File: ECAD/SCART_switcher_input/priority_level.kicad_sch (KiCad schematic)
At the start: 4 parts, among them U4 74LVC1G04, U5 74LVC1G08, U6 74LVC1G08

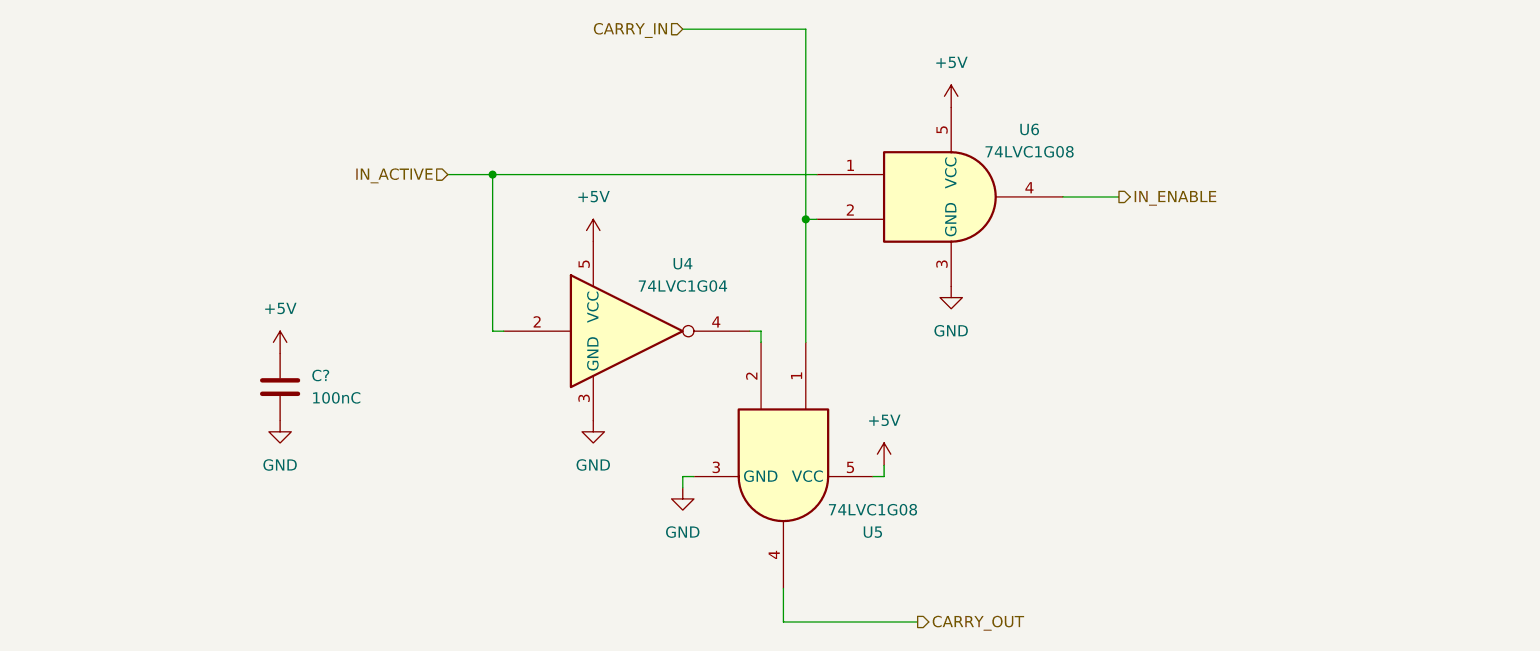
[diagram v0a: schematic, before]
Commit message: Progressed ECAD.
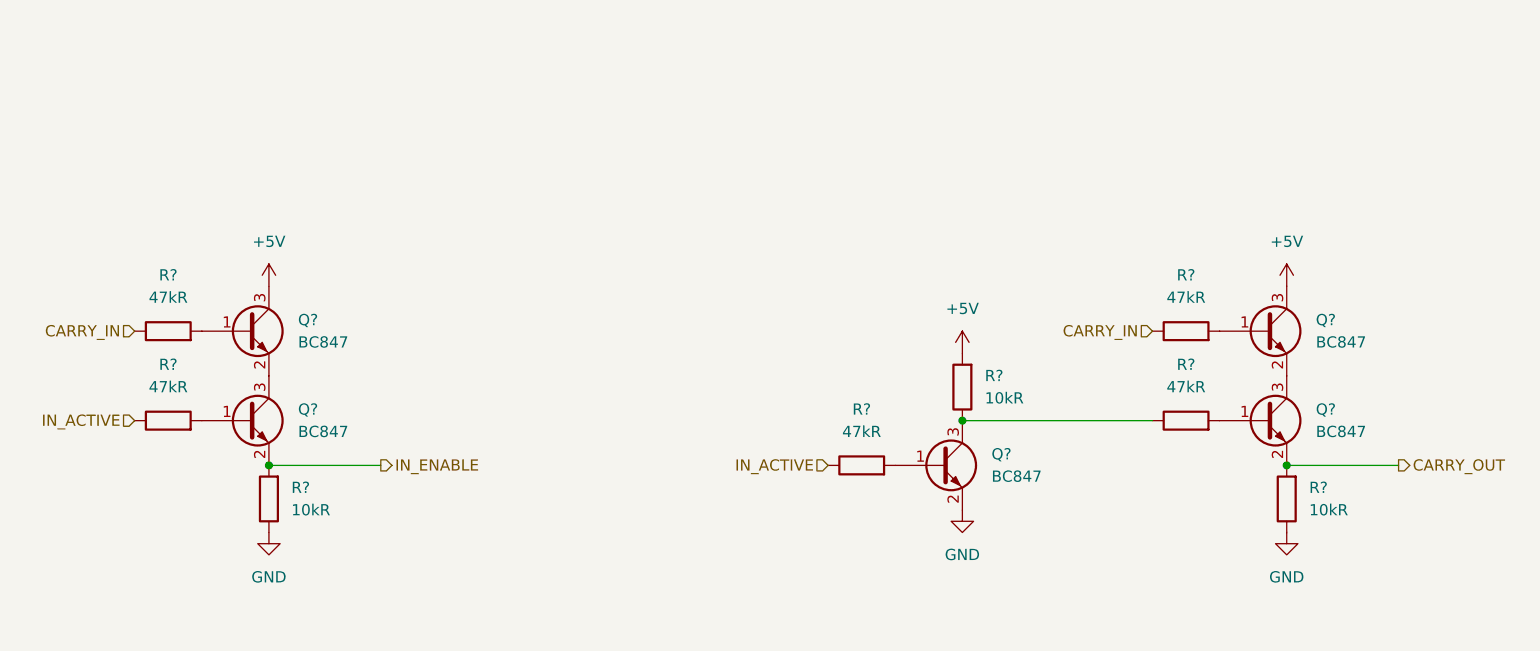
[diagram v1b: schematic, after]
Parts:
- removed C?: 100nC, Capacitor_SMD:C_0805_2012Metric, symbol Device:C
- removed U4: 74LVC1G04, Package_TO_SOT_SMD:SOT-353_SC-70-5, symbol 74xGxx:74AHC1G04
- removed U5, U6: 74LVC1G08, Package_TO_SOT_SMD:SOT-353_SC-70-5, symbol 74xGxx:74AHC1G08
- added Q? (x5): BC847, Package_TO_SOT_SMD:SOT-23, symbol Transistor_BJT:BC847
- added R? (x5): 47kR, Resistor_SMD:R_0805_2012Metric, symbol Device:R
- added R? (x3): 10kR, Resistor_SMD:R_0805_2012Metric, symbol Device:R
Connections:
- net +5V: now also Q?.3 (C), Q?.3 (C), R?.2
- net CARRY_IN: now also R?.1, R?.1
- net CARRY_OUT: now also Q?.2 (E), R?.2
- net GND: now also Q?.2 (E), R?.1, R?.1
- net IN_ACTIVE: now also R?.1, R?.1
- net IN_ENABLE: now also Q?.2 (E), R?.2
- new net: Q?.1 (B), R?.2 (x5)
- new net: Q?.2 (E), Q?.3 (C) (x2)
- new net: Q?.3 (C), R?.1, R?.1

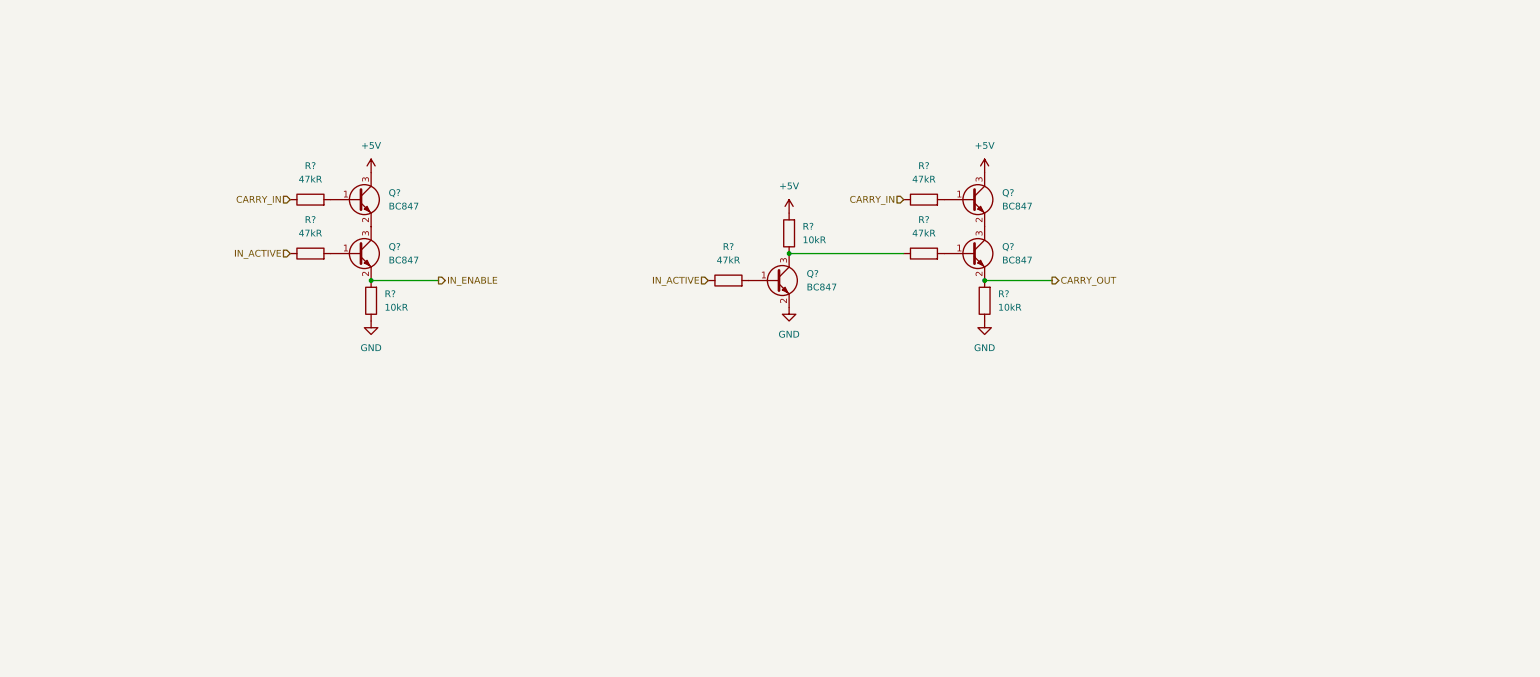
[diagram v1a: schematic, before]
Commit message: Progressed ECAD.
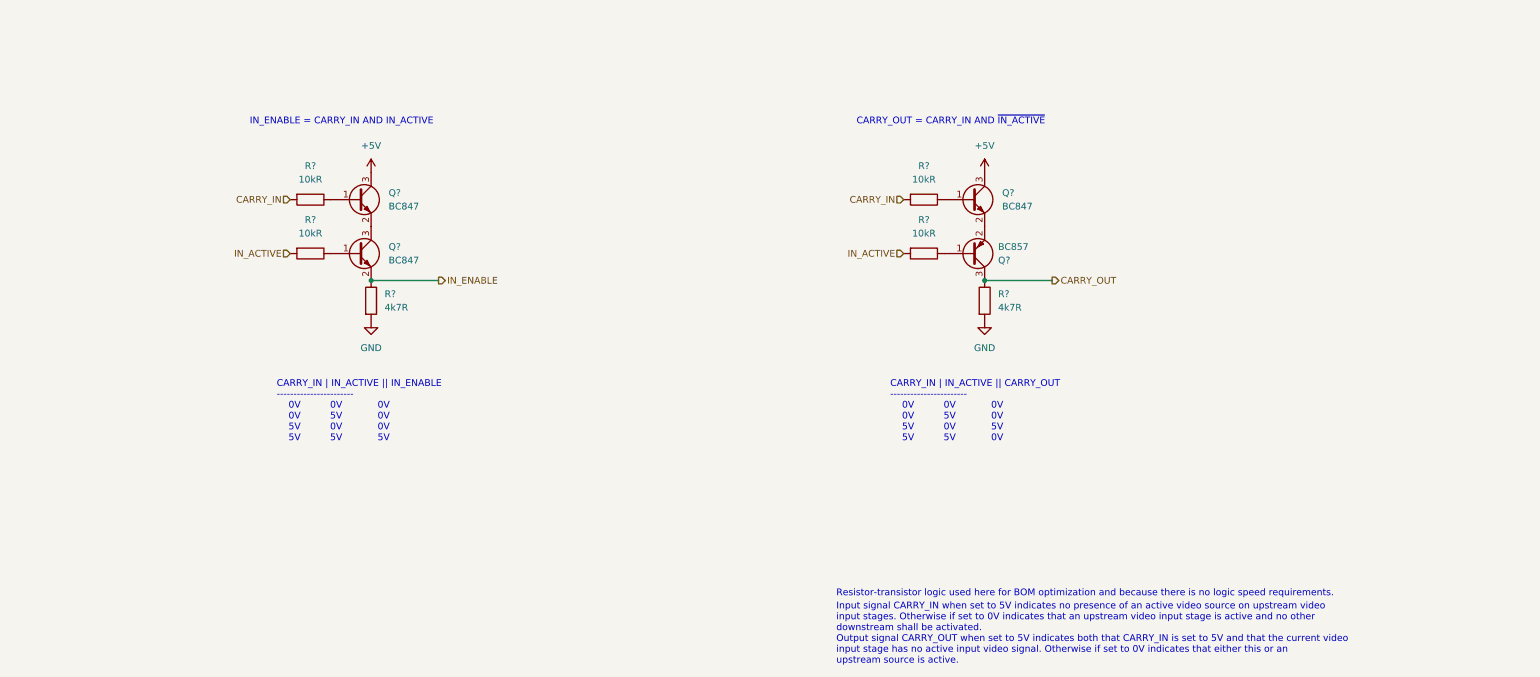
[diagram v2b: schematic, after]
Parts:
- removed Q? (x2): BC847, Package_TO_SOT_SMD:SOT-23, symbol Transistor_BJT:BC847
- removed R? (x5): 47kR, Resistor_SMD:R_0805_2012Metric, symbol Device:R
- removed R? (x3): 10kR, Resistor_SMD:R_0805_2012Metric, symbol Device:R
- added Q?: BC857, Package_TO_SOT_SMD:SOT-23, symbol Transistor_BJT:BC857
- added R? (x2): 4k7R, Resistor_SMD:R_0805_2012Metric, symbol Device:R
- added R? (x4): 10kR, Resistor_SMD:R_0805_2012Metric, symbol Device:R
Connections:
- net CARRY_IN: now also R?.2, R?.2
- net CARRY_OUT: now also Q?.3 (C), R?.1
- net GND: now also R?.2, R?.2
- net IN_ACTIVE: now also R?.2, R?.2
- net IN_ENABLE: now also R?.1
- net at Q?.1 (B): now also R?.1 (x3)
- net at Q?.2 (E): now also Q?.2 (E)
- new net: Q?.1 (B), R?.1
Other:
- note added: "CARRY_IN | IN_ACTIVE || CARRY_OUT ----------------------- 0V 0V 0V 0V 5V 0V 5V 0V 5V 5V 5V 0V"
- note added: "CARRY_IN | IN_ACTIVE || IN_ENABLE ----------------------- 0V 0V 0V 0V 5V 0V 5V 0V 0V 5V 5V 5V"
- note added: "CARRY_OUT = CARRY_IN AND ~{IN_ACTIVE}"
- note added: "IN_ENABLE = CARRY_IN AND IN_ACTIVE"
- note added: "Input signal CARRY_IN when set to 5V indicates no presence of an active video source on upstream video input stages. Otherwise if set to 0V indicates that an upstream video input stage is active and no other downstream shall be activated. Output signal CARRY_OUT when set to 5V indicates both that CARRY_IN is set to 5V and that the current video input stage has no active input video signal. Otherw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"
- note added: "Resistor-transistor logic used here for BOM optimization and because there is no logic speed requirements."

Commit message: progressed ecad.
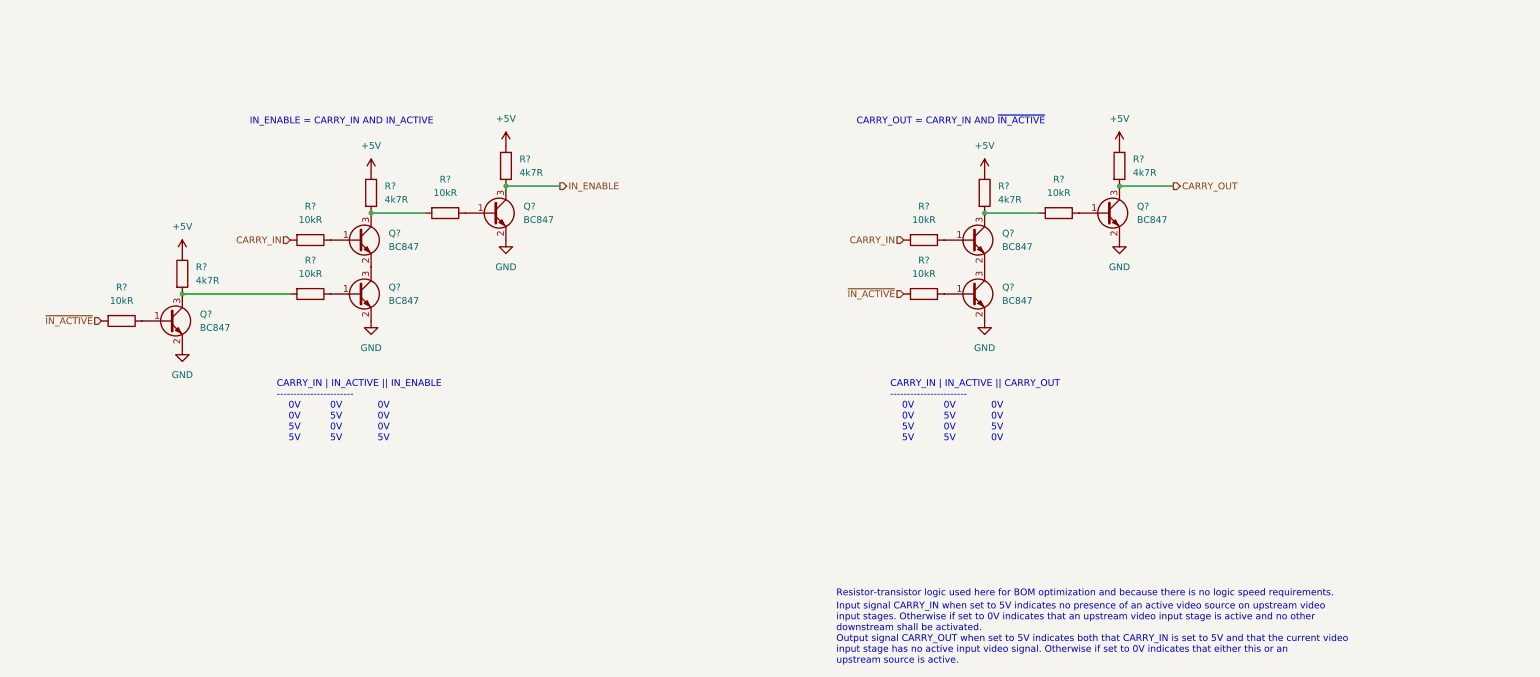
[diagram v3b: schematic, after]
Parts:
- removed Q?: BC857, Package_TO_SOT_SMD:SOT-23, symbol Transistor_BJT:BC857
- removed R? (x2): 4k7R, Resistor_SMD:R_0805_2012Metric, symbol Device:R
- added Q? (x4): BC847, Package_TO_SOT_SMD:SOT-23, symbol Transistor_BJT:BC847
- added R? (x5): 4k7R, Resistor_SMD:R_0805_2012Metric, symbol Device:R
- added R? (x3): 10kR, Resistor_SMD:R_0805_2012Metric, symbol Device:R
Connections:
- net +5V: now also R?.1, R?.1, R?.1, R?.1, R?.1; no longer Q?.3 (C), Q?.3 (C)
- net CARRY_OUT: now also Q?.3 (C), R?.2
- net GND: now also Q?.2 (E), Q?.2 (E), Q?.2 (E), Q?.2 (E), Q?.2 (E)
- net IN_ENABLE: now also Q?.3 (C), R?.2; no longer Q?.2 (E)
- net at Q?.2 (E): now also Q?.3 (C)
- net at R?.1: now also Q?.1 (B)
- net IN_ACTIVE: no longer names the net of R?.2
- net IN_ACTIVE: now also Q?.3 (C), R?.2; no longer R?.2
- new net: Q?.3 (C), R?.2, R?.2 (x2)
- new net: Q?.1 (B), R?.1 (x3)
- new net ~{IN_ACTIVE}: R?.2, R?.2
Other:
- moved on the sheet: Q?, R?
